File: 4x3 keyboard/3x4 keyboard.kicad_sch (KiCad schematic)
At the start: 33 parts, among them J1 Groove, SW1 SW_Push, SW10 SW_Push, SW11 SW_Push, SW12 SW_Push, SW2 SW_Push, SW3 SW_Push, SW4 SW_Push, SW5 SW_Push, SW6 SW_Push, SW7 SW_Push, SW8 SW_Push, SW9 SW_Push, U1 TCA8418, U2 MCP1700x-330xxTT

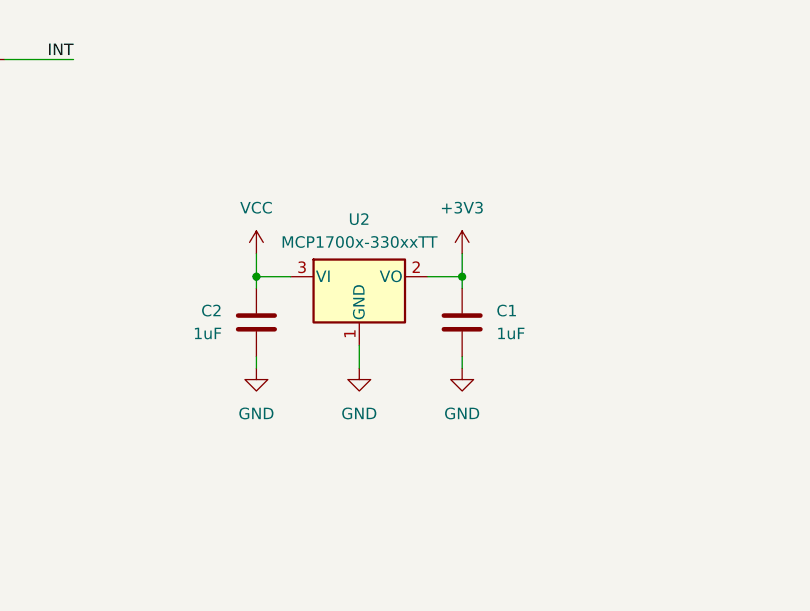
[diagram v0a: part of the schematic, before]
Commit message: Finishing touches and a readme
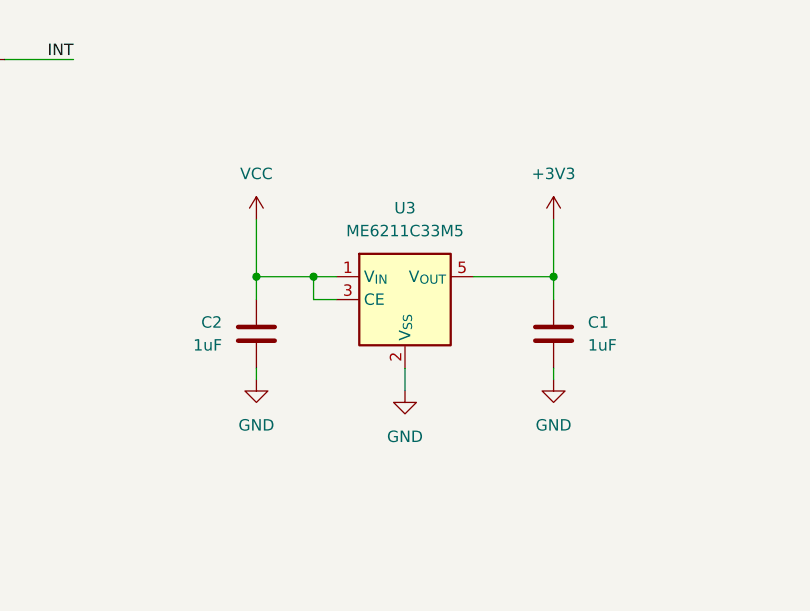
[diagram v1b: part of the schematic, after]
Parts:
- removed U2: MCP1700x-330xxTT, Package_TO_SOT_SMD:SOT-23, symbol Regulator_Linear:MCP1700x-330xxTT
- added U3: ME6211C33M5, Package_TO_SOT_SMD:SOT-23-5, symbol Regulator_Linear:ME6211C33M5
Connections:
- net +3V3: now also U3.5 (V_{OUT})
- net GND: now also U3.2 (V_{SS})
- net VCC: now also U3.1 (V_{IN}), U3.3 (CE)
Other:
- moved on the sheet: C1, C2
